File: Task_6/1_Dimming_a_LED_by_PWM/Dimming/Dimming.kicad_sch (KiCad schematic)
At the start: 6 parts, among them Q1 IC=0.5 VCEO=45

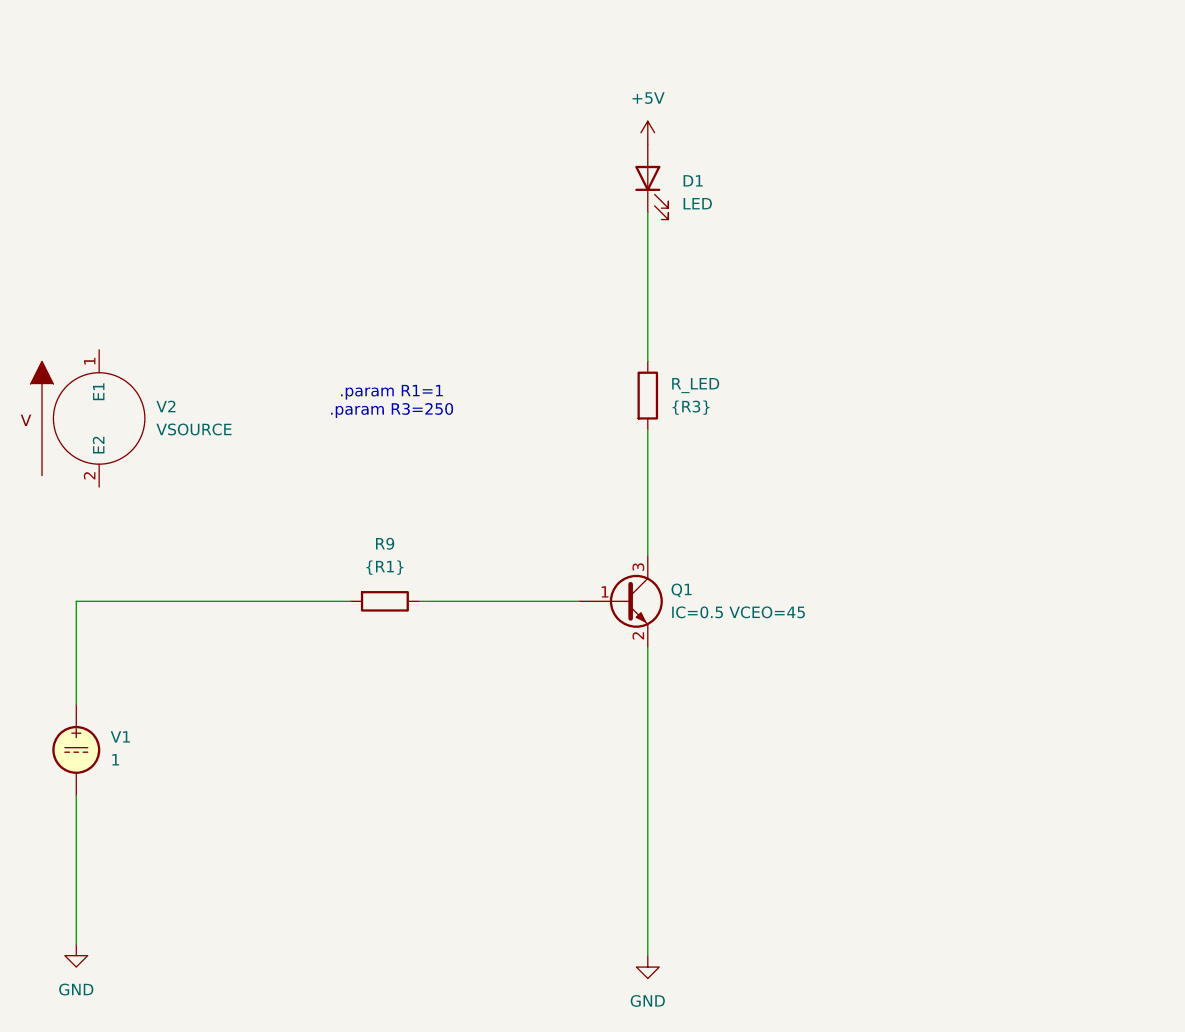
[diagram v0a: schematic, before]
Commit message: Expanded 6
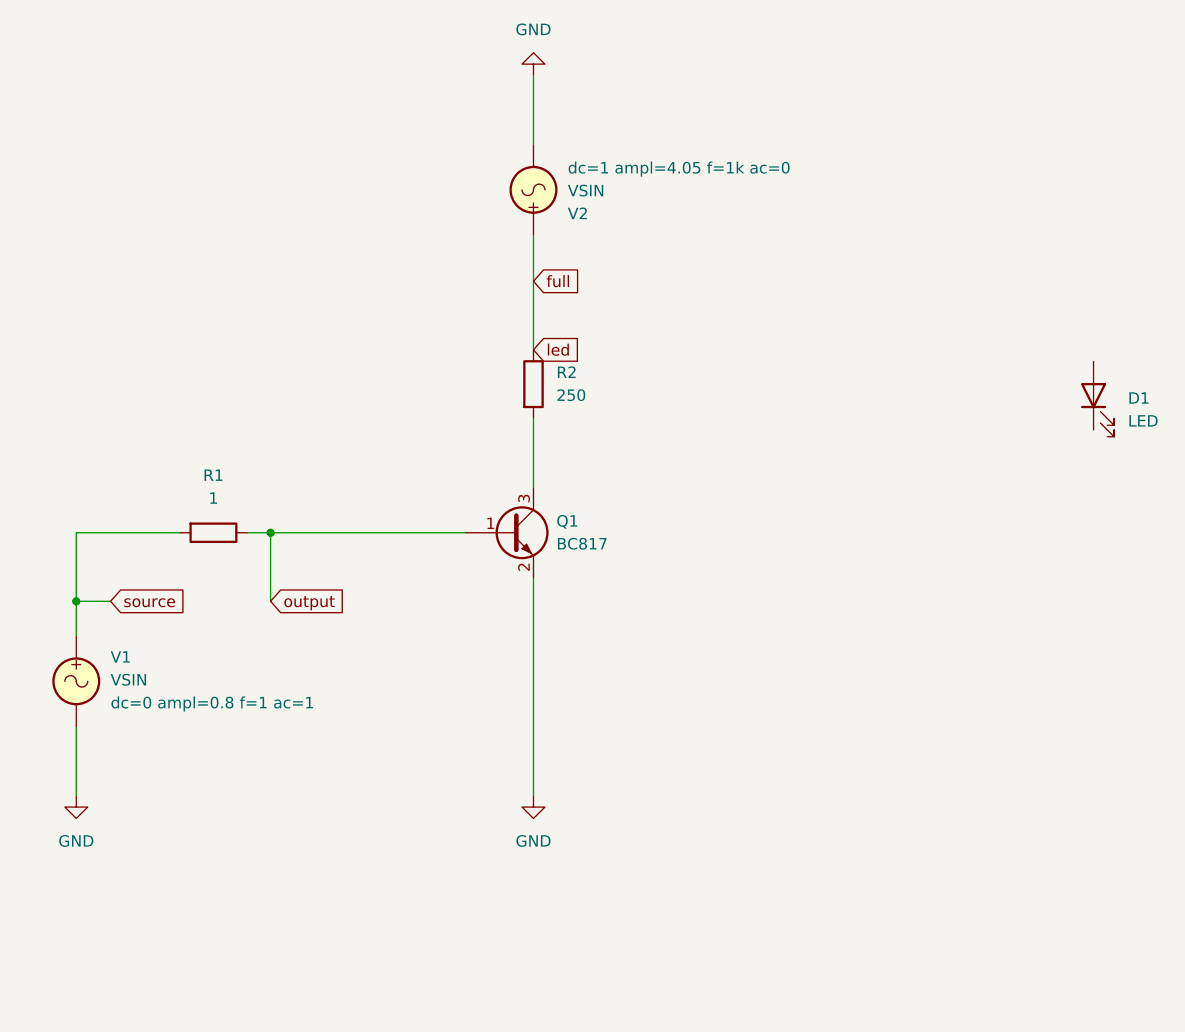
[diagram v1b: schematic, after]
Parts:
- removed R9: {R1}, symbol Device:R
- removed R_LED: {R3}, symbol Device:R
- removed V1: 1, symbol Simulation_SPICE:VDC
- removed V2: VSOURCE, symbol pspice:VSOURCE
- added R1: 1, symbol Device:R
- added R2: 250, symbol Device:R
- added V1, V2: VSIN, symbol Simulation_SPICE:VSIN
- Q1: value IC=0.5 VCEO=45 -> BC817
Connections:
- net GND: now also V1.2, V2.2
- net output: now reaches Q1.1 (B)
- net output: now also R1.1
- net at Q1.3 (C): now also R2.2
- net +5V: no longer names the net of D1.2 (A)
- new net full: R2.1, V2.1
- new net source: R1.2, V1.1
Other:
- note removed: ".param R1=1 .param R3=250"
